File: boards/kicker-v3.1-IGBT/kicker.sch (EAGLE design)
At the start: 134 parts, among them J1 B2PS-VH(LF)(SN), J2 HFW8R-1ST, J3 B2PS-VH(LF)(SN), J4 B2PS-VH(LF)(SN), J5 2-PIN_2MM-H, J6 3-PIN_2MM-H, J7 !BTN_KCK_PRE_EXT, J8 !BTN_CHP_PRE_EXT, J9 !BTN_CHG_PRE_EXT, Q1 ATP302ATPAK, Q10 BSS806NSOT-23-3, Q2 IRFS4227, Q3 BSS127, Q4 BSS127, Q5 BSS127, Q6 BSS127, Q7 AOD1N60, U1 R-78E5.0-0.5, U2 15V, U3 LT3751FE, U4 AT32ATQFP44, U5 IX4427N, U6 MAX6817, U7 MAX6817

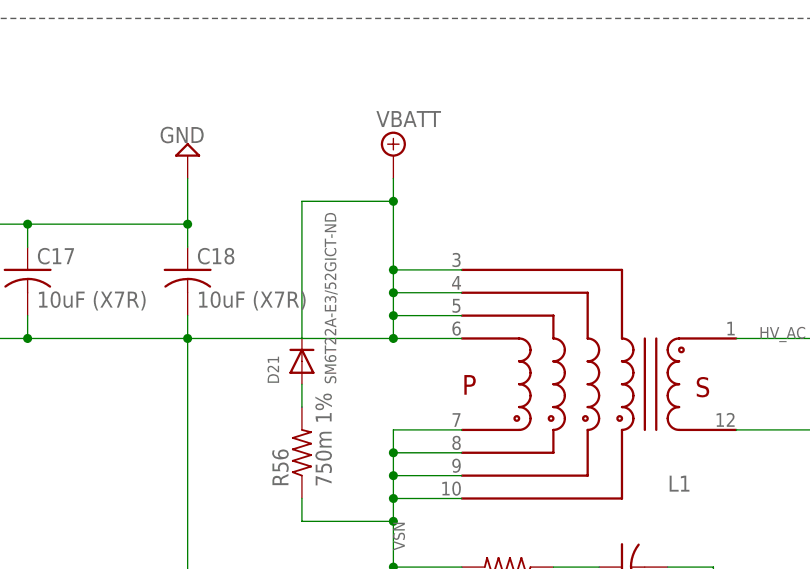
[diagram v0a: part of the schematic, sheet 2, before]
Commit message: Minor Fixes
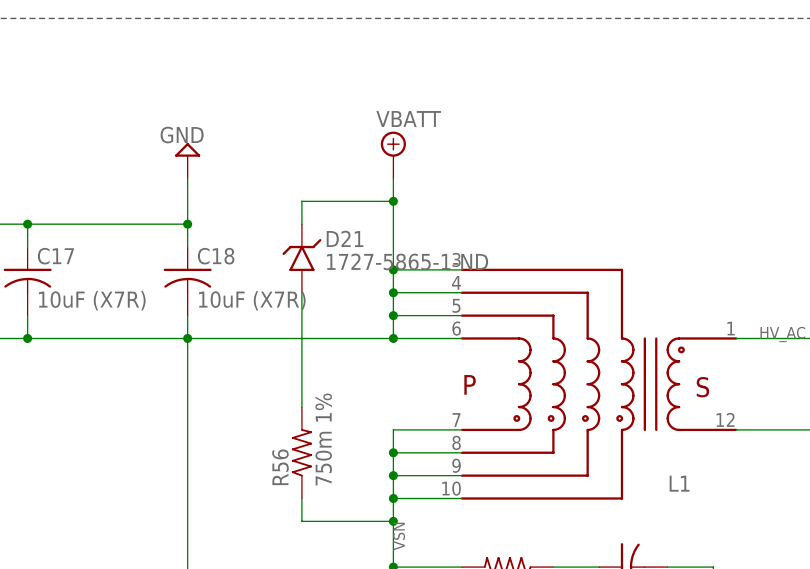
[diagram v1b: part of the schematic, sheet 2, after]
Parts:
- D21: value SM6T22A-E3/52GICT-ND -> 1727-5865-1-ND; device adafruit:DIODESOD-123 -> RoboJackets-Diodes:TVS
